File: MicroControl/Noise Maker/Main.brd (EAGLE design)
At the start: 22.9 x 24.8 mm, 16 parts, among them IC1 STM8L151G6U6, IC2 317EMP, Q1 BSS123, X1 MKDSN1,5/2-5,08, X2 MKDSN1,5/2-5,08

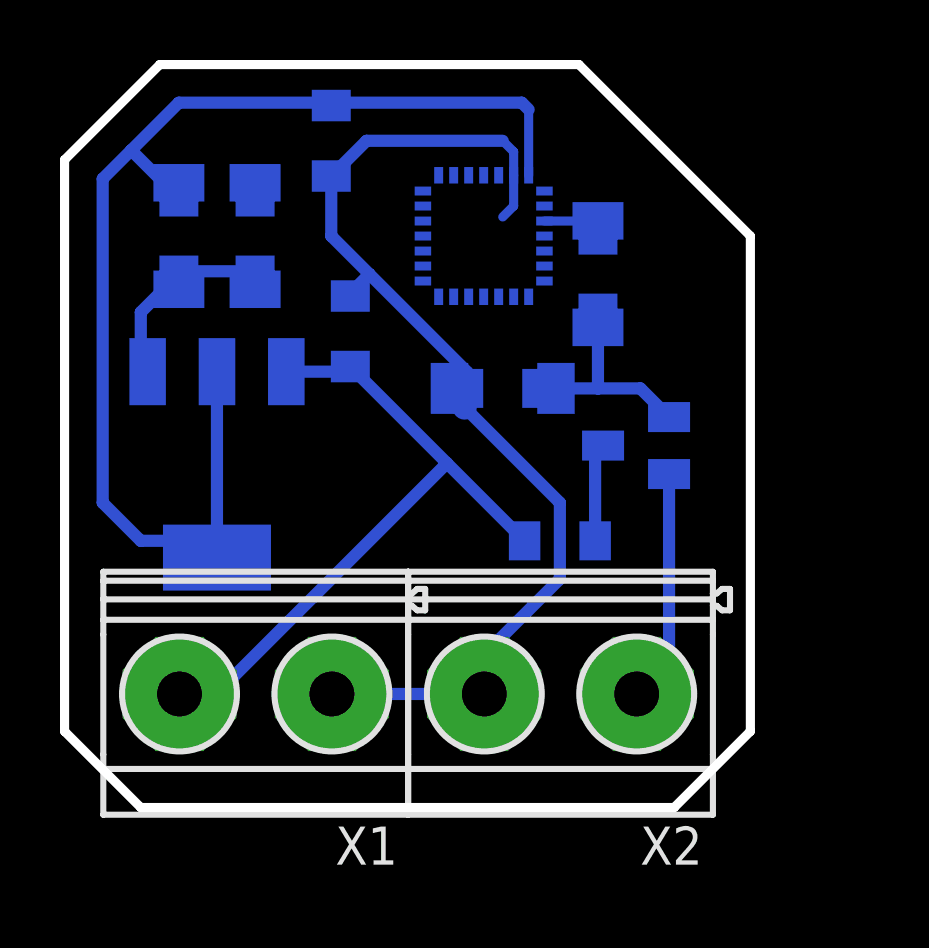
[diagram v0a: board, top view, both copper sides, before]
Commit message: Тщшыу
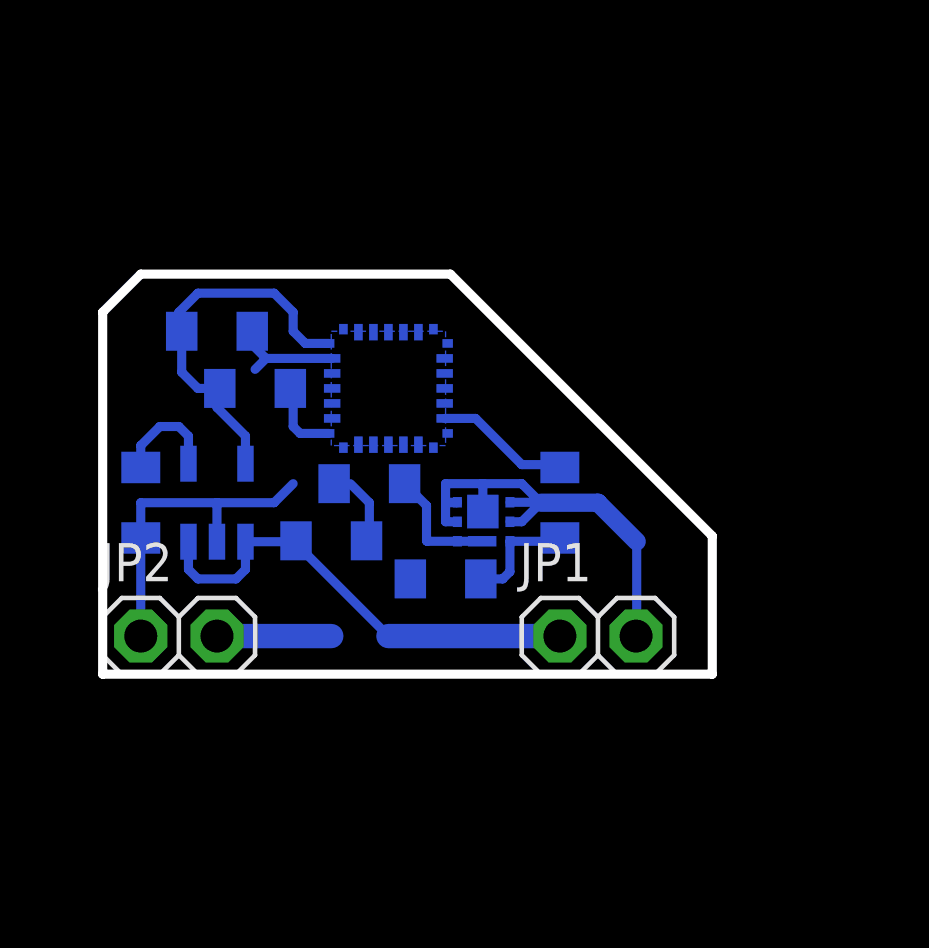
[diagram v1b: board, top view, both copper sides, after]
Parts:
- removed IC2: 317EMP, linear:SOT223
- removed R3, R8: (no value), rcl:R0805
- removed R4, R5, R6: (no value), rcl:R1206
- removed R9: 680R, rcl:R0805
- removed X1, X2: MKDSN1,5/2-5,08, con-phoenix-508:MKDSN1,5/2-5,08
- added C3, C4: 10n, rcl:C0805
- added IC3: TS520533, v-reg:SOT25
- added JP1, JP2: (no value), pinhead:1X02
- C1, C2: value (none) -> 10u
- IC1: value STM8L151G6U6 -> STM8L151X4/6G6U6; device Namenlos:QFPN28 -> Namenlos:QFN28
- Q1: value BSS123 -> (none); device transistor-small-signal:SOT23 -> Namenlos:POWERFLAT-2X2
- R1, R2: device rcl:R0805 -> Namenlos:R0805
- R7: device rcl:R1206 -> Namenlos:R0805
- moved R2 10.4 mm to (10.2, 9.53), turned to 180 degrees
- moved R1 7.73 mm to (16.5, 8.89)
- moved C2 7.41 mm to (5.08, 14.6), turned to 180 degrees
- moved C1 7.01 mm to (8.89, 7.62), turned to 180 degrees
- moved R7 6.63 mm to (12.7, 6.35)
- moved IC1 5.99 mm to (10.8, 12.7), turned to 180 degrees
- moved Q1 5.68 mm to (14.0, 8.26)
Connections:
- removed net N$10: Q1.3, R9.1
- removed net N$11: Q1.2, X2.1
- new net N$13: JP2.2
- new net N$2: C3.1, IC3.4
- new net N$7: Q1.S, Q1.S4, R2.2
- new net N$9: JP1.2, Q1.D, Q1.D1, Q1.D2, Q1.D5, Q1.D6
- net GND: now also C3.2, IC3.2, JP2.1, R2.1; no longer R3.1, R5.1, R8.1, X1.1, X2.2
- net N$1: now also IC1.20; no longer IC1.10, R6.2
- net N$3: now also C4.1, IC1.1; no longer IC2.1, R2.1, R3.2, R4.1, R5.2
- net N$4: now also C4.2, IC3.5; no longer IC2.4, R2.2, R4.2
- net N$8: now also Q1.G3; no longer Q1.1, R6.1, R8.2
- net VCC: now also IC3.1, IC3.3, JP1.1; no longer IC2.3, R9.2, X1.2
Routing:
- net N$4: track 43.4 -> 12.8 mm
- net GND: track 38.2 -> 17.1 mm
- net N$9: track 0.00 -> 16.0 mm
- net N$11: track 7.78 -> 0.00 mm
- net VCC: track 22.5 -> 15.9 mm
- net N$3: track 7.40 -> 2.60 mm
- net N$7: track 0.00 -> 4.07 mm
- net N$13: track 0.00 -> 3.81 mm
- net N$2: track 0.00 -> 3.64 mm
- net N$8: track 7.40 -> 3.79 mm
- net N$10: track 3.28 -> 0.00 mm
- net N$1: track 2.39 -> 4.52 mm
- added copper zone on layer 16, net N$6
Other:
- board size 22.9 x 24.8 mm -> 20.3 x 13.3 mm

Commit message: _
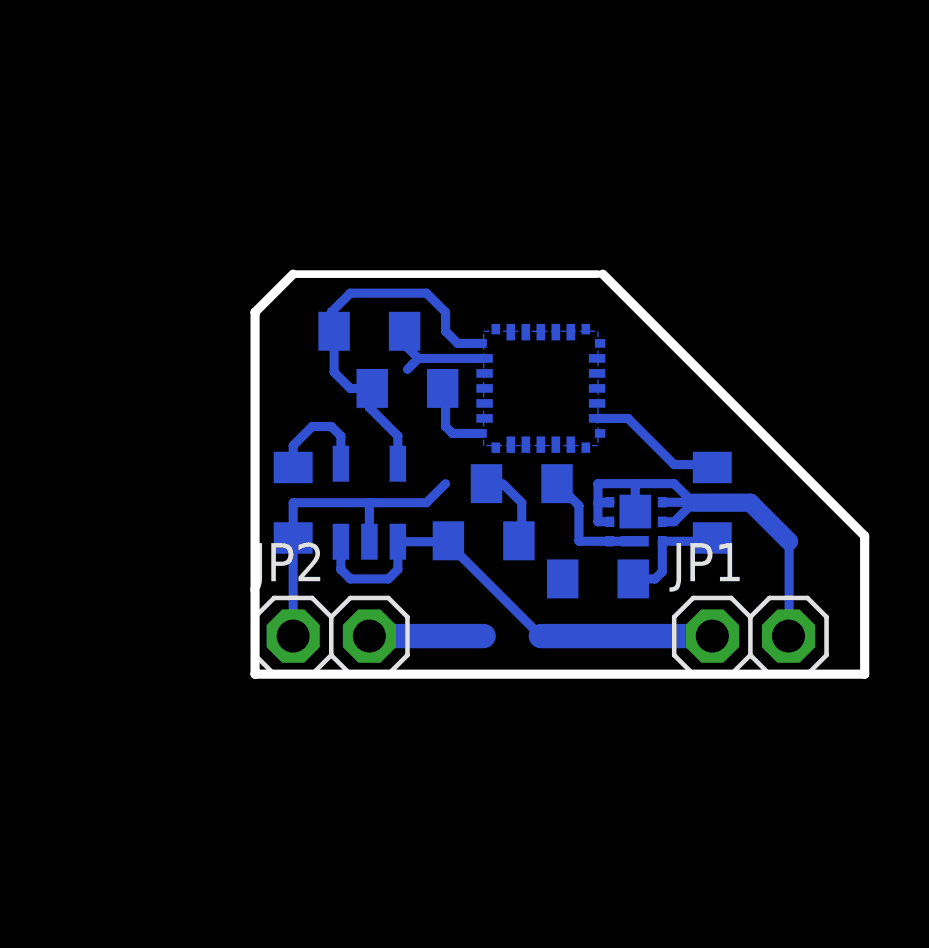
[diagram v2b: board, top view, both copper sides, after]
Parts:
- moved R7 5.08 mm to (17.8, 6.35)
- moved C1 5.08 mm to (14.0, 7.62)
- moved C2 5.08 mm to (10.2, 14.6)
- moved C3 5.08 mm to (7.62, 8.89)
- moved C4 5.08 mm to (11.4, 12.7)
- moved IC1 5.08 mm to (15.9, 12.7)
- moved IC3 5.08 mm to (10.2, 8.89)
- moved JP2 5.08 mm to (8.89, 4.45)
- moved Q1 5.08 mm to (19.1, 8.26)
- moved R2 5.08 mm to (15.2, 9.53)
- moved JP1 5.08 mm to (22.9, 4.45)
- moved R1 5.08 mm to (21.6, 8.89)
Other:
- outline, holes or cut-outs redrawn
